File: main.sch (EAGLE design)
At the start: 31 parts, among them IC1 ATMEGA328P-PU, IC2 LM7805, J1 2,1mm, Q1 16 MHz

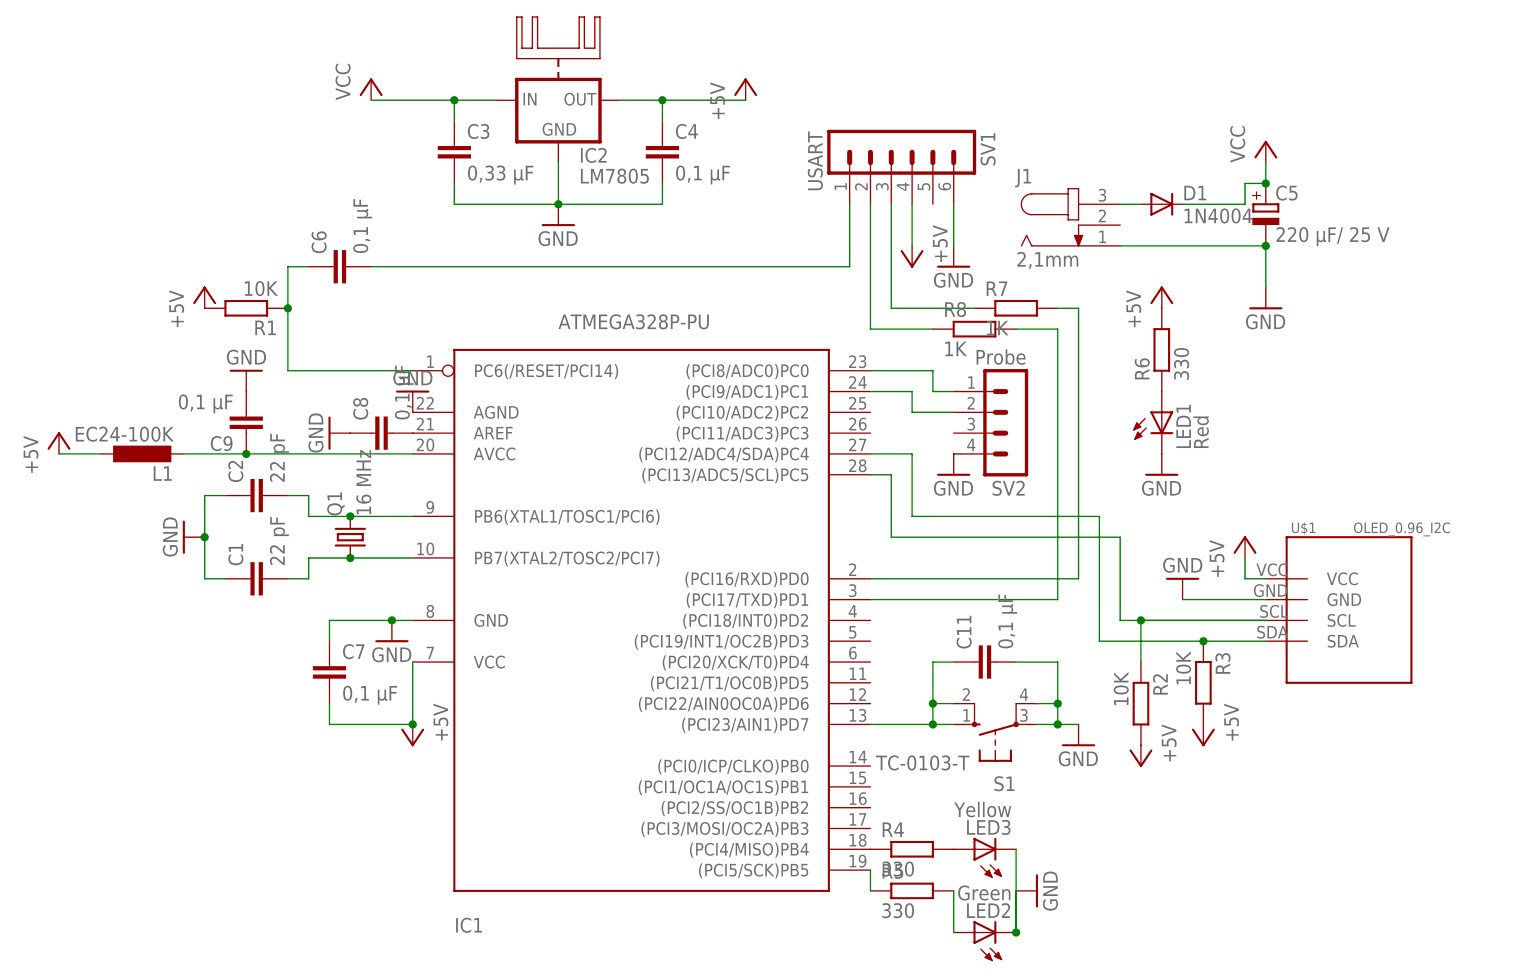
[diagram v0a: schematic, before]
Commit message: Opravy na celorepublikové kolo
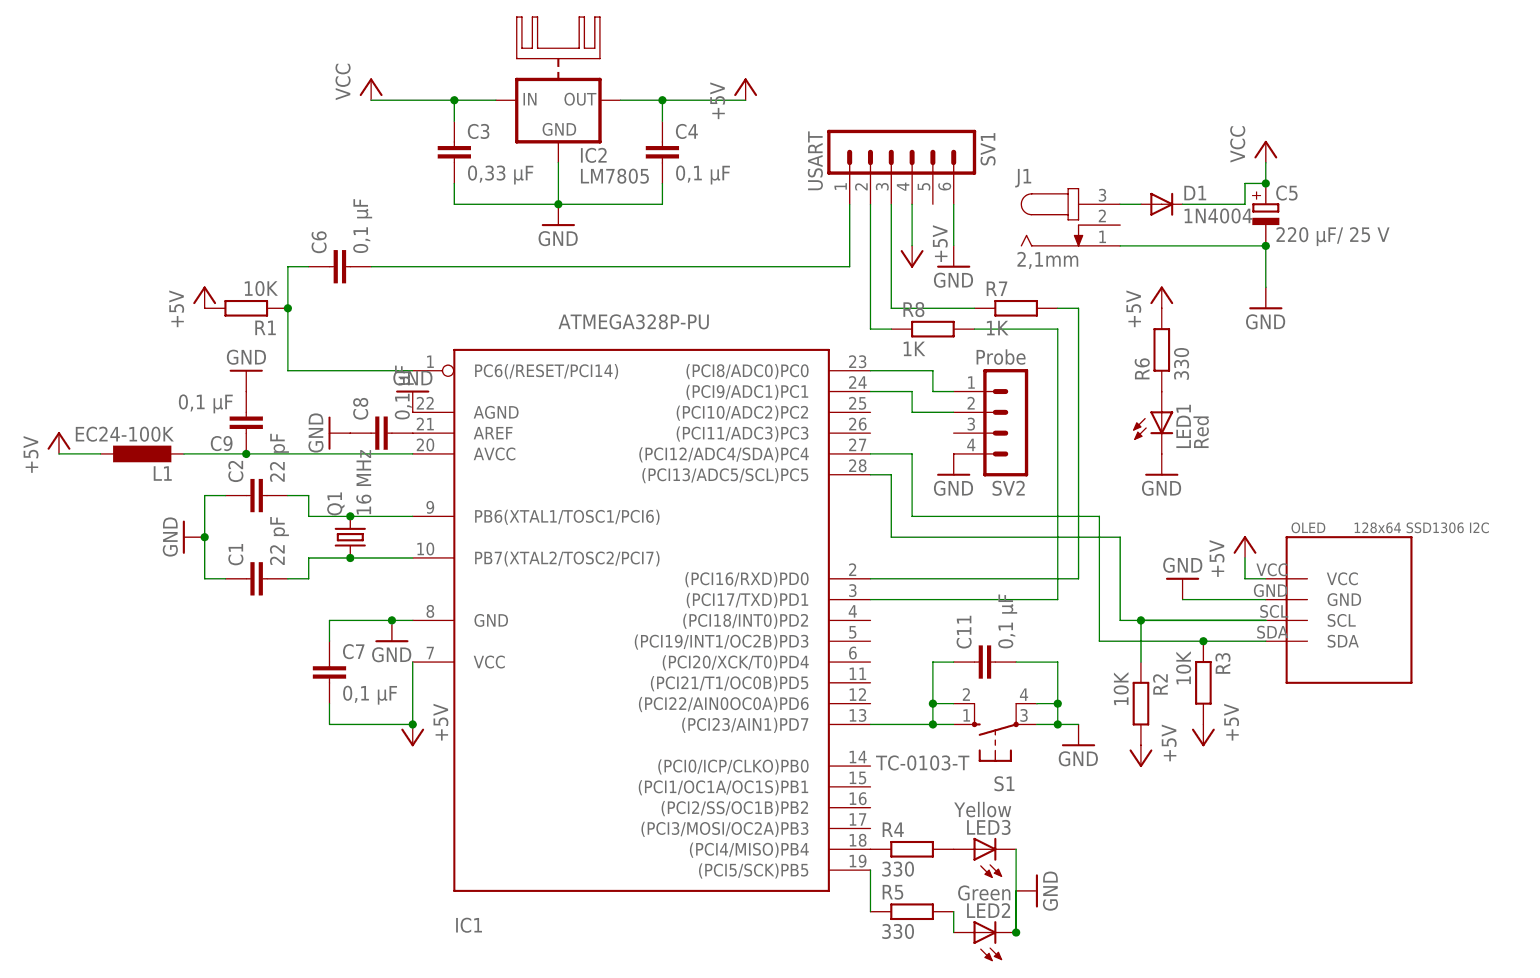
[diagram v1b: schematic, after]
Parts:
- OLED: value OLED_0.96_I2C -> 128x64 SSD1306 I2C
- renumbered U$1 to OLED
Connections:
- net N$13 renamed IJVCC
- net N$4 renamed SCL
- net N$6 renamed BTN
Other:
- moved on the sheet: R5, R8
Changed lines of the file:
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@@
 <?xml version="1.0" encoding="utf-8"?>
 <!DOCTYPE eagle SYSTEM "eagle.dtd">
-<eagle version="8.2.0">
+<eagle version="8.2.1">
 <drawing>
 <settings>
@@
 <part name="C6" library="rcl" library_urn="urn:adsk.eagle:library:334" deviceset="C-EU" device="050-025X075" value="0,1 μF"/>
 <part name="P+6" library="supply1" library_urn="urn:adsk.eagle:library:371" deviceset="VCC" device=""/>
-<part name="U$1" library="tft_1.8_1.44_oled_0.96" deviceset="OLED_0.96_I2C" device=""/>
+<part name="OLED" library="tft_1.8_1.44_oled_0.96" deviceset="OLED_0.96_I2C" device="" value="128x64 SSD1306 I2C"/>
 <part name="IC2" library="78xx_with_heatsink" deviceset="78XXH" device="" value="LM7805"/>
 <part name="GND7" library="supply1" library_urn="urn:adsk.eagle:library:371" deviceset="GND" device=""/>
@@
 <instance part="C6" gate="G$1" x="73.66" y="104.14" rot="R90"/>
 <instance part="P+6" gate="VCC" x="187.96" y="119.38"/>
-<instance part="U$1" gate="G$1" x="198.12" y="60.96" rot="R270"/>
+<instance part="OLED" gate="G$1" x="198.12" y="60.96" rot="R270"/>
 <instance part="IC2" gate="A" x="101.6" y="124.46"/>
 <instance part="GND7" gate="1" x="83.82" y="88.9" rot="R180"/>
@@
 <instance part="LED3" gate="G$1" x="152.4" y="33.02" rot="R90"/>
 <instance part="R4" gate="G$1" x="144.78" y="33.02"/>
-<instance part="R5" gate="G$1" x="144.78" y="27.94"/>
+<instance part="R5" gate="G$1" x="144.78" y="25.4"/>
 <instance part="GND12" gate="1" x="160.02" y="27.94" rot="R90"/>
 <instance part="R6" gate="G$1" x="175.26" y="93.98" rot="R90"/>
@@
 <instance part="GND13" gate="1" x="175.26" y="78.74"/>
 <instance part="R7" gate="G$1" x="157.48" y="99.06"/>
-<instance part="R8" gate="G$1" x="152.4" y="96.52"/>
+<instance part="R8" gate="G$1" x="147.32" y="96.52"/>
 </instances>
 <busses>
@@
 <pinref part="GND5" gate="1" pin="GND"/>
 <wire x1="187.96" y1="63.5" x2="177.8" y2="63.5" width="0.1524" layer="91"/>
-<pinref part="U$1" gate="G$1" pin="GND"/>
+<pinref part="OLED" gate="G$1" pin="GND"/>
 </segment>
 <segment>
@@
 <wire x1="187.96" y1="66.04" x2="185.42" y2="66.04" width="0.1524" layer="91"/>
 <wire x1="185.42" y1="66.04" x2="185.42" y2="68.58" width="0.1524" layer="91"/>
-<pinref part="U$1" gate="G$1" pin="VCC"/>
+<pinref part="OLED" gate="G$1" pin="VCC"/>
 </segment>
 <segment>
@@
 <wire x1="167.64" y1="73.66" x2="167.64" y2="58.42" width="0.1524" layer="91"/>
 <wire x1="167.64" y1="58.42" x2="180.34" y2="58.42" width="0.1524" layer="91"/>
-<pinref part="U$1" gate="G$1" pin="SDA"/>
+<pinref part="OLED" gate="G$1" pin="SDA"/>
 <wire x1="180.34" y1="58.42" x2="187.96" y2="58.42" width="0.1524" layer="91"/>
 <wire x1="144.78" y1="81.28" x2="144.78" y2="73.66" width="0.1524" layer="91"/>
@@
 </segment>
 </net>
-<net name="N$4" class="0">
+<net name="SCL" class="0">
 <segment>
 <pinref part="IC1" gate="G$1" pin="(PCI13/ADC5/SCL)PC5"/>
@@
 <wire x1="142.24" y1="78.74" x2="142.24" y2="71.12" width="0.1524" layer="91"/>
 <wire x1="142.24" y1="71.12" x2="170.18" y2="71.12" width="0.1524" layer="91"/>
-<pinref part="U$1" gate="G$1" pin="SCL"/>
+<pinref part="OLED" gate="G$1" pin="SCL"/>
 <wire x1="170.18" y1="60.96" x2="172.72" y2="60.96" width="0.1524" layer="91"/>
 <pinref part="R2" gate="G$1" pin="1"/>
@@
 <wire x1="162.56" y1="63.5" x2="139.7" y2="63.5" width="0.1524" layer="91"/>
 <pinref part="R8" gate="G$1" pin="2"/>
-<wire x1="162.56" y1="96.52" x2="157.48" y2="96.52" width="0.1524" layer="91"/>
-</segment>
-</net>
-<net name="N$6" class="0">
+<wire x1="162.56" y1="96.52" x2="152.4" y2="96.52" width="0.1524" layer="91"/>
+</segment>
+</net>
+<net name="BTN" class="0">
 <segment>
 <pinref part="IC1" gate="G$1" pin="(PCI23/AIN1)PD7"/>
@@
 </segment>
 </net>
-<net name="N$13" class="0">
+<net name="IJVCC" class="0">
 <segment>
 <pinref part="J1" gate="G$1" pin="3"/>
@@
 <pinref part="IC1" gate="G$1" pin="(PCI5/SCK)PB5"/>
 <pinref part="R5" gate="G$1" pin="1"/>
-<wire x1="139.7" y1="27.94" x2="139.7" y2="30.48" width="0.1524" layer="91"/>
+<wire x1="139.7" y1="25.4" x2="139.7" y2="30.48" width="0.1524" layer="91"/>
 </segment>
 </net>
@@
 <pinref part="R5" gate="G$1" pin="2"/>
 <pinref part="LED2" gate="G$1" pin="A"/>
-<wire x1="149.86" y1="22.86" x2="149.86" y2="27.94" width="0.1524" layer="91"/>
+<wire x1="149.86" y1="22.86" x2="149.86" y2="25.4" width="0.1524" layer="91"/>
 </segment>
 </net>
@@
 <wire x1="139.7" y1="111.76" x2="139.7" y2="96.52" width="0.1524" layer="91"/>
 <pinref part="R8" gate="G$1" pin="1"/>
-<wire x1="147.32" y1="96.52" x2="139.7" y2="96.52" width="0.1524" layer="91"/>
+<wire x1="142.24" y1="96.52" x2="139.7" y2="96.52" width="0.1524" layer="91"/>
 </segment>
 </net>
@@
 </sheet>
 </sheets>
+<errors>
+</errors>
 </schematic>
 </drawing>
